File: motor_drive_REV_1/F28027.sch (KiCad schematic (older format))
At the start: 34 parts, among them J4 Conn_01x06, J5 Conn_01x06, U8 TMS20F28027PTT-custom

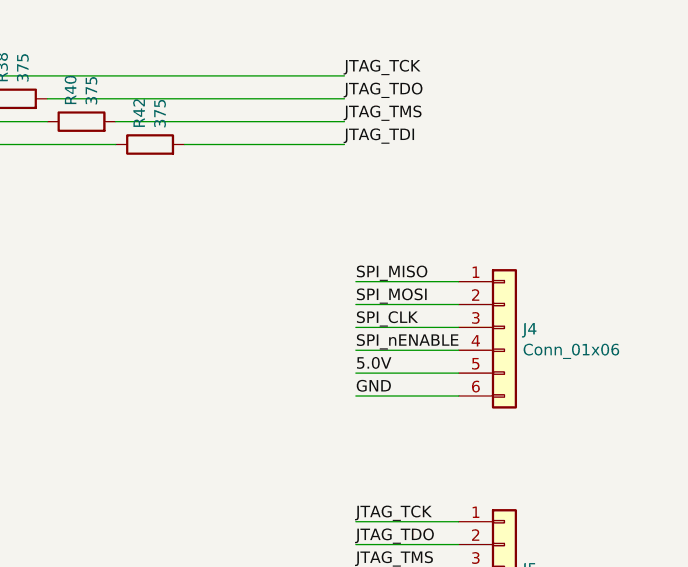
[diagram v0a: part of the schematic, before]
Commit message: layout
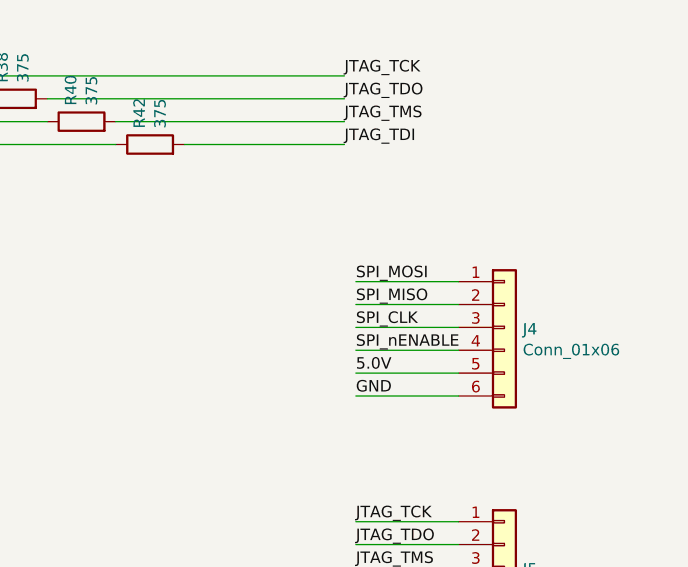
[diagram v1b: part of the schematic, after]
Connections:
- net SPI_MISO: now also J4.2 (Pin_2); no longer J4.1 (Pin_1)
- net SPI_MOSI: now also J4.1 (Pin_1); no longer J4.2 (Pin_2)
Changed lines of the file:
@@
 GND
 Text Label 12450 5450 0    50   ~ 0
+SPI_MOSI
+Text Label 12450 5550 0    50   ~ 0
 SPI_MISO
-Text Label 12450 5550 0    50   ~ 0
-SPI_MOSI
 Text Label 12450 5650 0    50   ~ 0
 SPI_CLK
